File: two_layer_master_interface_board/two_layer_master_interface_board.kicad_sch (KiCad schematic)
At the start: 12 parts, among them J1 USB_C_Receptacle_USB2.0_16P, J2 Conn_01x06_Socket, U1 FT232RL, U2 THVD1450DR, U3 RP2040

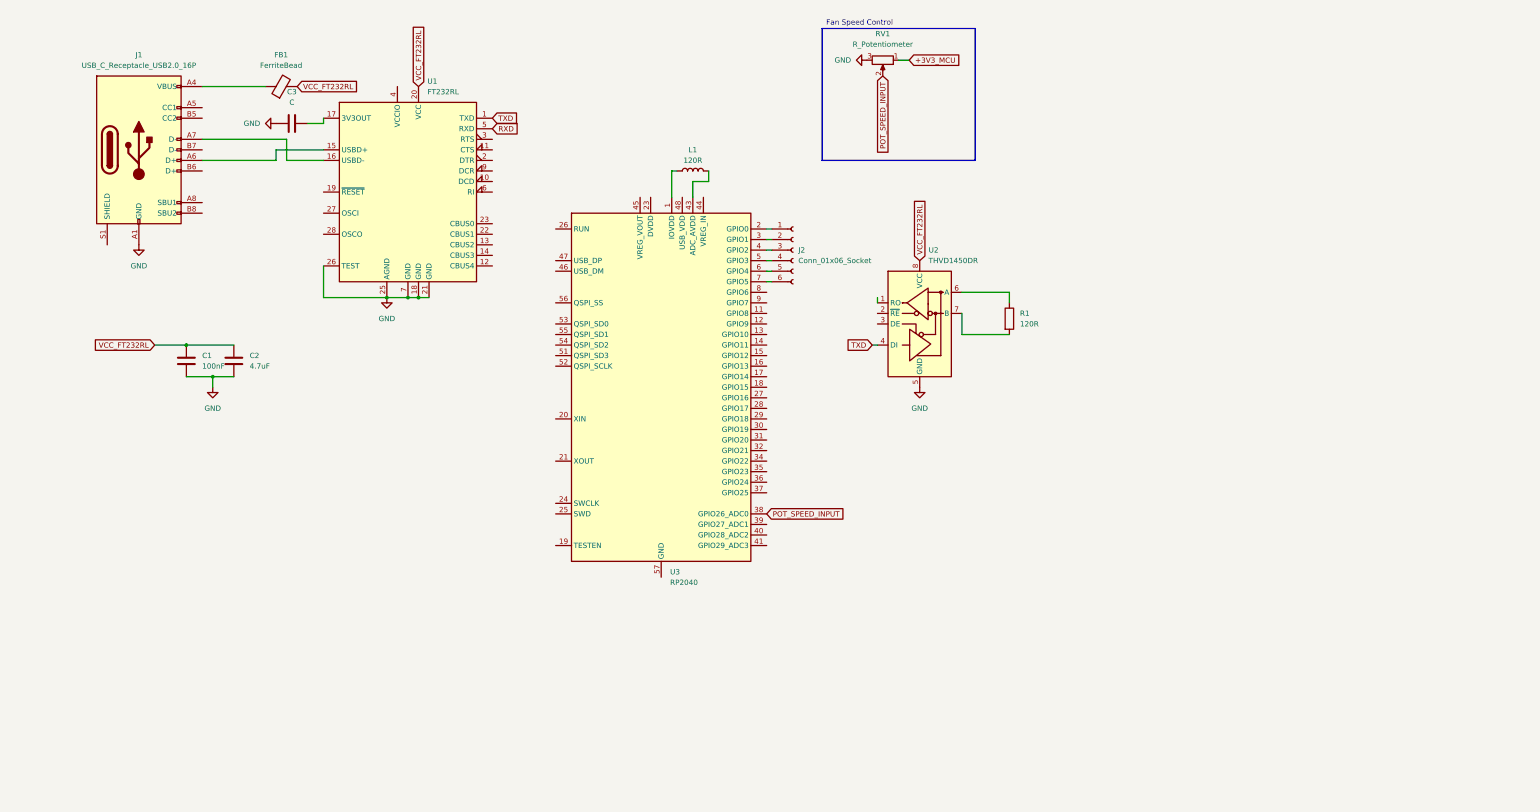
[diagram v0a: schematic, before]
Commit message: AI question for next phase of the project
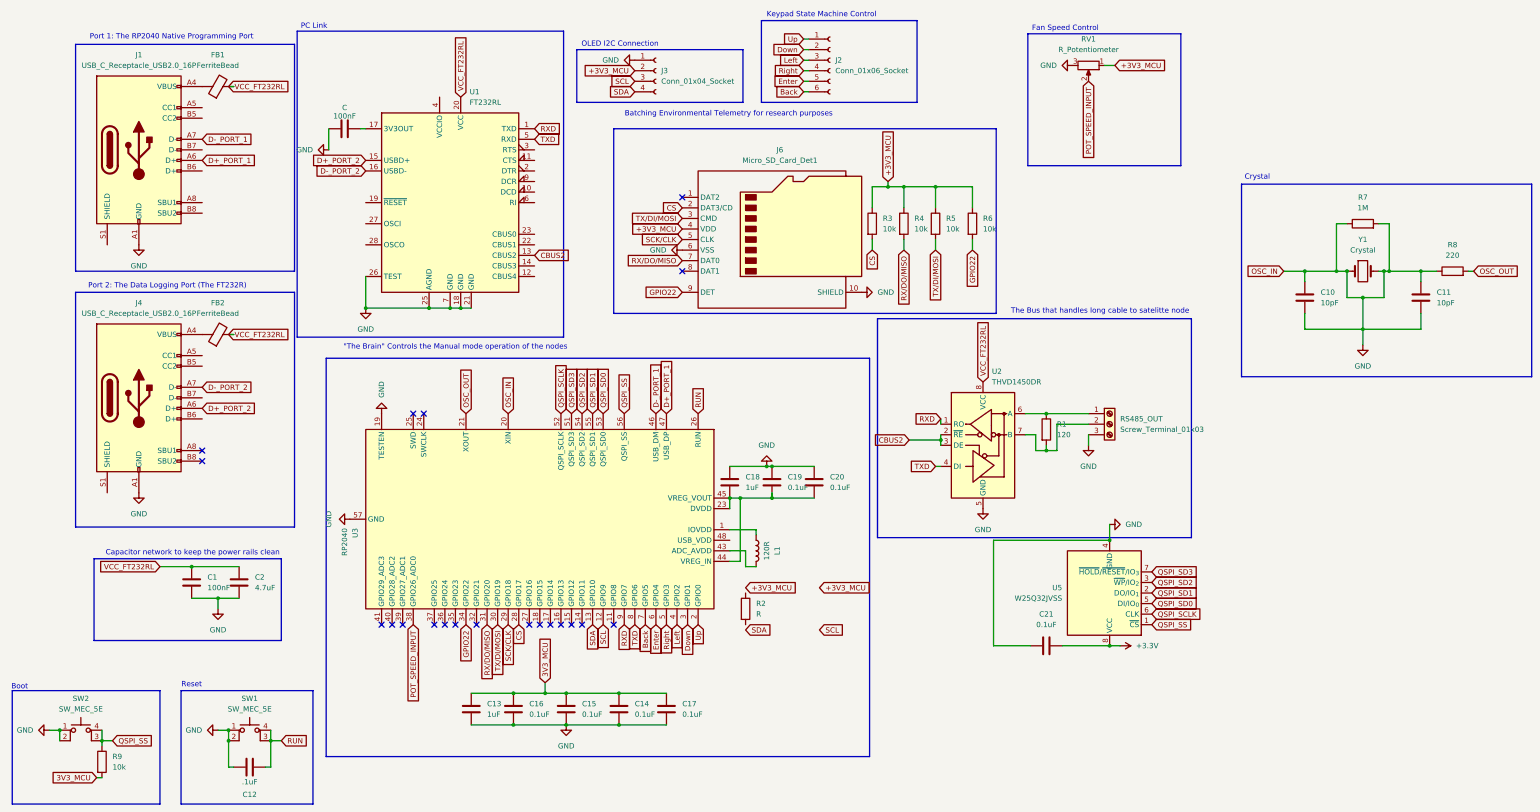
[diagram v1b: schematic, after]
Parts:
- added C10, C11: 10pF, symbol Device:C
- added C12: .1uF, symbol Device:C
- added C13, C18: 1uF, symbol Device:C
- added C14, C15, C16, C17, C19, C20, C21: 0.1uF, symbol Device:C
- added FB2: FerriteBead, symbol Device:FerriteBead
- added J3: Conn_01x04_Socket, symbol Connector:Conn_01x04_Socket
- added J4: USB_C_Receptacle_USB2.0_16P, symbol Connector:USB_C_Receptacle_USB2.0_16P
- added J6: Micro_SD_Card_Det1, symbol Connector:Micro_SD_Card_Det1
- added R2: R, symbol Device:R
- added R3, R4, R5, R6, R9: 10k, symbol Device:R
- added R7: 1M, symbol Device:R
- added R8: 220, symbol Device:R
- added RS485_OUT: Screw_Terminal_01x03, symbol Connector:Screw_Terminal_01x03
- added SW1, SW2: SW_MEC_5E, symbol Switch:SW_MEC_5E
- added U5: W25Q32JVSS, Package_SO:SOIC-8_5.3x5.3mm_P1.27mm, symbol Memory_Flash:W25Q32JVSS
- added Y1: Crystal, symbol Device:Crystal
- R1: value 120R -> 120
- renumbered C3 to 100nF
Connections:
- net +3V3_MCU: now also J3.2 (Pin_2), J6.4 (VDD), R3.1, R4.1, R5.1, R6.1
- net GND: now also U3.19 (TESTEN), U3.20 (XIN), U3.57 (GND), C10.1, C10.2, C11.1, C11.2, C12.1, C13.2, C14.2, C15.2, C16.2, C17.2, C18.1, C19.1, C20.1, C21.1, J3.1 (Pin_1), J4.A1 (GND), J4.A12 (GND), J4.B1 (GND), J4.B12 (GND), J6.10 (SHIELD), J6.6 (VSS), R7.1, R7.2, R8.1, RS485_OUT.3 (Pin_3), SW1.1, SW1.2, SW2.1, SW2.2, U5.4 (GND), Y1.1, Y1.2
- net RXD: now also U1.1 (TXD), U2.1 (RO), U3.9 (GPIO7); no longer U1.5 (RXD)
- net TXD: now also U1.5 (RXD), U3.8 (GPIO6); no longer U1.1 (TXD)
- net VCC_FT232RL: now also FB2.2
- net CBUS2: now reaches U1.13 (CBUS2)
- net CBUS2: now also U2.2 (~{RE}), U2.3 (DE)
- net D+_PORT_1: now reaches J1.A6 (D+)
- net D+_PORT_1: now also U3.47 (USB_DP); no longer U1.15 (USBD+)
- net D-_PORT_1: now reaches J1.A7 (D-)
- net D-_PORT_1: now also U3.46 (USB_DM); no longer U1.16 (USBD-)
- net Up: now reaches J2.1 (Pin_1), U3.2 (GPIO0)
- net Down: now reaches J2.2 (Pin_2), U3.3 (GPIO1)
- net Left: now reaches J2.3 (Pin_3), U3.4 (GPIO2)
- net Right: now reaches J2.4 (Pin_4), U3.5 (GPIO3)
- net Enter: now reaches J2.5 (Pin_5), U3.6 (GPIO4)
- net Back: now reaches J2.6 (Pin_6), U3.7 (GPIO5)
- net SCL: now reaches U3.12 (GPIO9)
- net SCL: now also J3.3 (Pin_3)
- net SDA: now reaches U3.13 (GPIO10)
- net SDA: now also J3.4 (Pin_4)
- net OSC_OUT: now reaches U3.21 (XOUT)
- net OSC_OUT: now also R8.2
- net at U3.23 (DVDD), U3.50 (DVDD): now also U3.44 (VREG_IN), U3.45 (VREG_VOUT), C18.2, C19.2, C20.2
- net RUN: now reaches U3.26 (RUN)
- net RUN: now also C12.2, SW1.3 (K), SW1.4 (A)
- net CS: now reaches U3.28 (GPIO17)
- net CS: now also J6.2 (DAT3/CD), R3.2
- net SCK/CLK: now reaches U3.29 (GPIO18)
- net SCK/CLK: now also J6.5 (CLK)
- net TX/DI/MOSI: now reaches U3.30 (GPIO19)
- net TX/DI/MOSI: now also J6.3 (CMD), R5.2
- net RX/DO/MISO: now reaches U3.31 (GPIO20)
- net RX/DO/MISO: now also J6.7 (DAT0), R4.2
- net GPIO22: now reaches U3.34 (GPIO22)
- net GPIO22: now also J6.9 (DET), R6.2
- net QSPI_SD3: now reaches U3.51 (QSPI_SD3)
- net QSPI_SD3: now also U5.7 (~{HOLD}/~{RESET}/IO_{3})
- net QSPI_SCLK: now reaches U3.52 (QSPI_SCLK)
- net QSPI_SCLK: now also U5.6 (CLK)
- net QSPI_SD0: now reaches U3.53 (QSPI_SD0)
- net QSPI_SD0: now also U5.5 (DI/IO_{0})
- net QSPI_SD2: now reaches U3.54 (QSPI_SD2)
- net QSPI_SD2: now also U5.3 (~{WP}/IO_{2})
- net QSPI_SD1: now reaches U3.55 (QSPI_SD1)
- net QSPI_SD1: now also U5.2 (DO/IO_{1})
- net QSPI_SS: now reaches U3.56 (QSPI_SS)
- net QSPI_SS: now also R9.1, SW2.3 (K), SW2.4 (A), U5.1 (~{CS})
- net at R1.1, U2.6 (A): now also RS485_OUT.1 (Pin_1)
- net at R1.2, U2.7 (B): now also RS485_OUT.2 (Pin_2)
- new net: FB2.1, J4.A4 (VBUS), J4.A9 (VBUS), J4.B4 (VBUS), J4.B9 (VBUS)
- new net +3.3V: C21.2, U5.8 (VCC)
- new net 3V3_MCU: C13.1, C14.1, C15.1, C16.1, C17.1, R9.2
- new net D+_PORT_2: J4.A6 (D+), U1.15 (USBD+)
- new net D-_PORT_2: J4.A7 (D-), U1.16 (USBD-)
- no-connect marks 0 -> 20
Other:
- note added: ""The Brain" Controls the Manual mode operation of the nodes"
- note added: "Batching Environmental Telemetry for research purposes"
- note added: "Boot"
- note added: "Capacitor network to keep the power rails clean"
- note added: "Crystal"
- note added: "Keypad State Machine Control"
- note added: "OLED I2C Connection"
- note added: "PC Link"
- note added: "Port 1: The RP2040 Native Programming Port"
- note added: "Port 2: The Data Logging Port (The FT232R)"
- note added: "Reset"
- note added: "The Bus that handles long cable to satelitte node"
- moved on the sheet: 100nF, C1, C2, FB1, J2, L1, RV1, U1, U2, U3

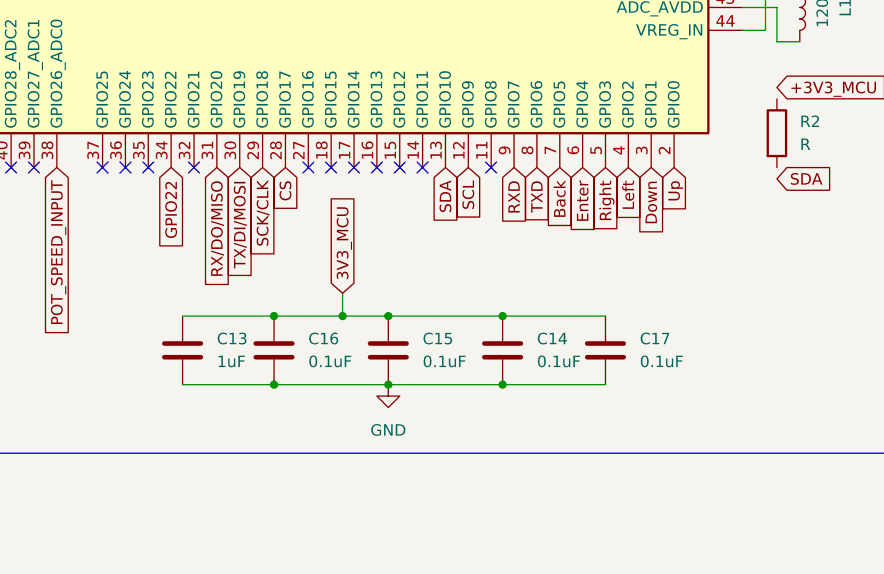
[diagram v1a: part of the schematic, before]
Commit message: arduino-nano-node-version
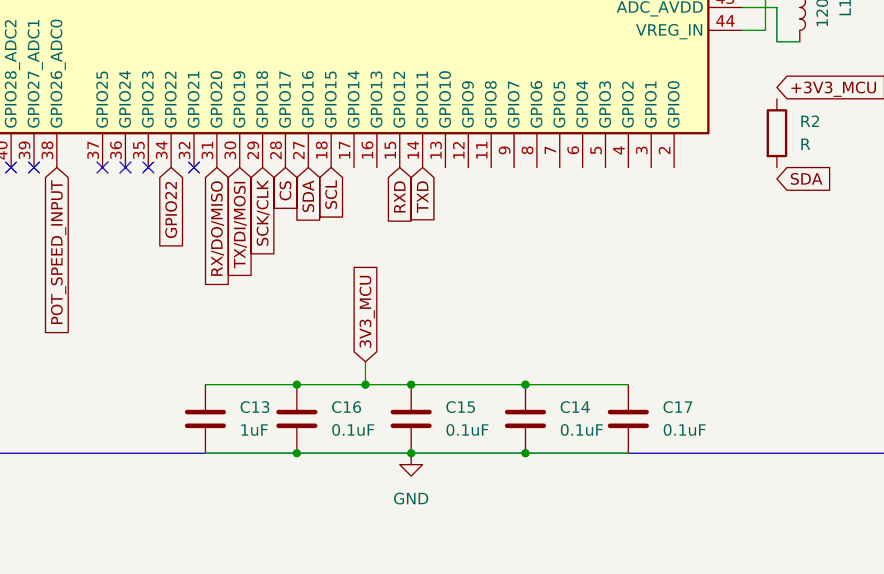
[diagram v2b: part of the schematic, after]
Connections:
- net Back: no longer U3.7 (GPIO5)
- net Down: no longer U3.3 (GPIO1)
- net Enter: no longer U3.6 (GPIO4)
- net Left: no longer U3.4 (GPIO2)
- net RXD: now also U3.15 (GPIO12); no longer U3.9 (GPIO7)
- net Right: no longer U3.5 (GPIO3)
- net SCL: now also U3.18 (GPIO15); no longer U3.12 (GPIO9)
- net SDA: now also U3.27 (GPIO16); no longer U3.13 (GPIO10)
- net TXD: now also U3.14 (GPIO11); no longer U3.8 (GPIO6)
- net Up: no longer U3.2 (GPIO0)
- no-connect marks 20 -> 13
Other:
- moved on the sheet: C13, C14, C15, C16, C17
